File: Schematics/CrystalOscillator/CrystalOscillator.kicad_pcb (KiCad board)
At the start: 2 copper layers, 8 parts, among them J1 Conn_01x24_Female, U1 74HC14, Y1 4MHz Crystal

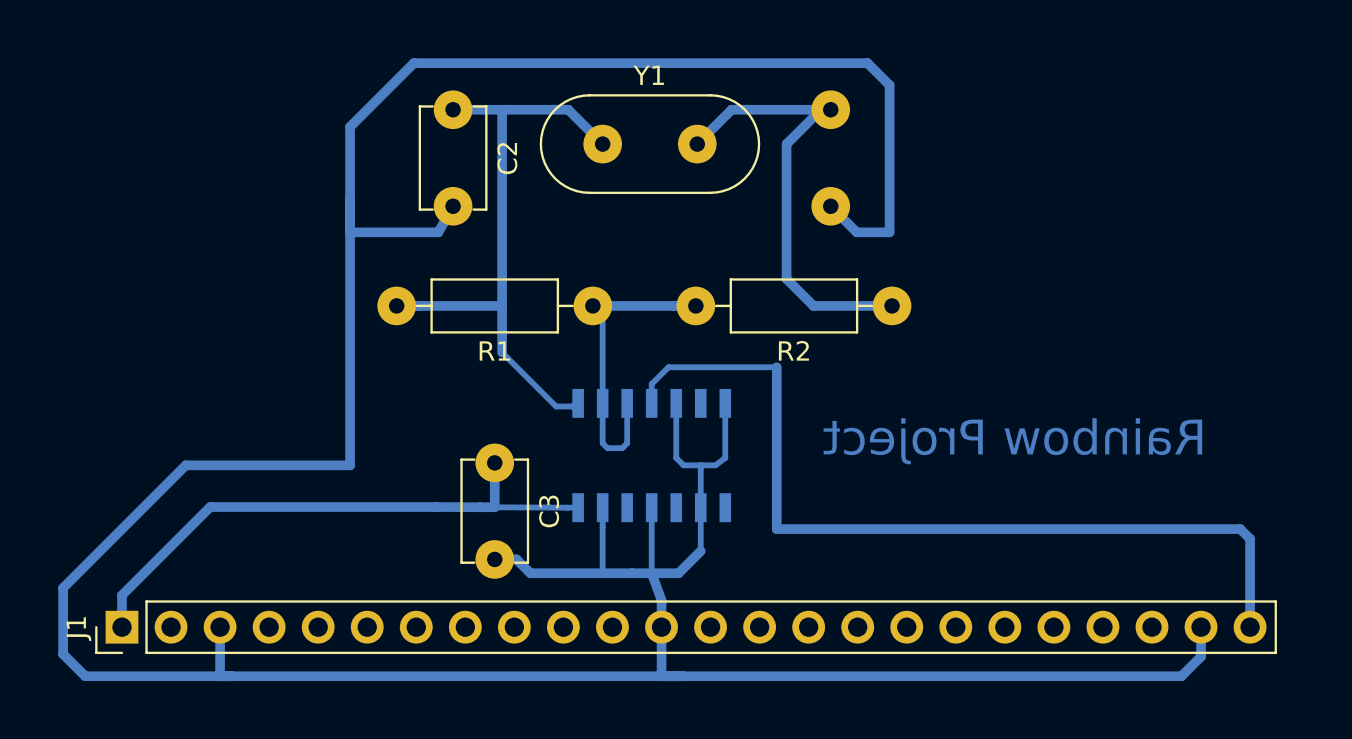
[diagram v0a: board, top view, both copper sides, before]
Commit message: Final version of 4 MHz clock PCB
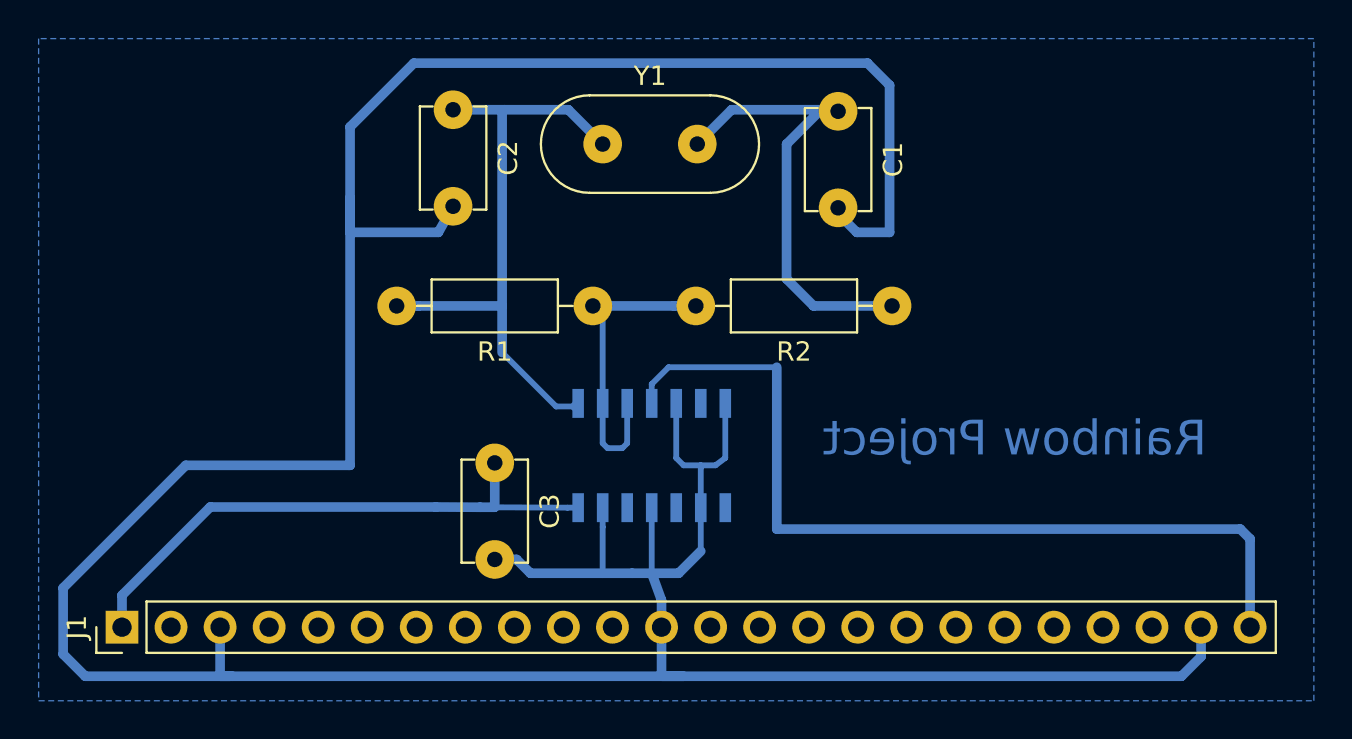
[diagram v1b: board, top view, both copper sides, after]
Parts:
- C1: moved to F.Cu
- moved C1 0.39 mm to (163.3, 104.1)
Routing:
- added copper zone on B.Cu, net GND
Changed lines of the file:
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@@
     (visible_elements 7FFFFFFF)
     (pcbplotparams
-      (layerselection 0x010fc_ffffffff)
+      (layerselection 0x00000_fffffffe)
       (usegerberextensions false)
       (usegerberattributes false)
@@
       (psa4output false)
       (plotreference true)
-      (plotvalue true)
-      (plotinvisibletext false)
+      (plotvalue false)
+      (plotinvisibletext true)
       (padsonsilk false)
       (subtractmaskfromsilk false)
-      (outputformat 1)
+      (outputformat 4)
       (mirror false)
       (drillshape 1)
       (scaleselection 1)
-      (outputdirectory ""))
+      (outputdirectory "D:/Data/Desktop/"))
   )
   (net 0 "")
@@
     )
   )
-  (module Capacitor_THT:C_Disc_D5.1mm_W3.2mm_P5.00mm (layer B.Cu)
-    (at 162.941 104.013 270)
+  (module Capacitor_THT:C_Disc_D5.1mm_W3.2mm_P5.00mm (layer F.Cu)
+    (at 163.322 104.093 270)
     (descr "C, Disc series, Radial, pin pitch=5.00mm, , diameter*width=5.1*3.2mm^2, Capacitor, http://www.vishay.com/docs/45233/krseries.pdf")
     (tags "C Disc series Radial pin pitch 5.00mm  diameter 5.1mm width 3.2mm Capacitor")
-    (fp_text reference C1 (at 2.5 2.85 270) (layer B.SilkS)
-      (effects (font (size 1 1) (thickness 0.15)) (justify mirror))
-    )
-    (fp_text value 3.3p (at 2.5 -2.85 270) (layer B.Fab)
-      (effects (font (size 1 1) (thickness 0.15)) (justify mirror))
-    )
-    (fp_line (start -0.05 1.6) (end -0.05 -1.6) (layer B.Fab) (width 0.1))
-    (fp_line (start -0.05 -1.6) (end 5.05 -1.6) (layer B.Fab) (width 0.1))
-    (fp_line (start 5.05 -1.6) (end 5.05 1.6) (layer B.Fab) (width 0.1))
-    (fp_line (start 5.05 1.6) (end -0.05 1.6) (layer B.Fab) (width 0.1))
-    (fp_line (start -0.17 1.721) (end 5.17 1.721) (layer B.SilkS) (width 0.12))
-    (fp_line (start -0.17 -1.721) (end 5.17 -1.721) (layer B.SilkS) (width 0.12))
-    (fp_line (start -0.17 1.721) (end -0.17 1.055) (layer B.SilkS) (width 0.12))
-    (fp_line (start -0.17 -1.055) (end -0.17 -1.721) (layer B.SilkS) (width 0.12))
-    (fp_line (start 5.17 1.721) (end 5.17 1.055) (layer B.SilkS) (width 0.12))
-    (fp_line (start 5.17 -1.055) (end 5.17 -1.721) (layer B.SilkS) (width 0.12))
-    (fp_line (start -1.05 1.85) (end -1.05 -1.85) (layer B.CrtYd) (width 0.05))
-    (fp_line (start -1.05 -1.85) (end 6.05 -1.85) (layer B.CrtYd) (width 0.05))
-    (fp_line (start 6.05 -1.85) (end 6.05 1.85) (layer B.CrtYd) (width 0.05))
-    (fp_line (start 6.05 1.85) (end -1.05 1.85) (layer B.CrtYd) (width 0.05))
-    (fp_text user %R (at 2.54 -0.381 270) (layer B.Fab)
-      (effects (font (size 1 1) (thickness 0.15)) (justify mirror))
+    (fp_text reference C1 (at 2.5 -2.85 270) (layer F.SilkS)
+      (effects (font (size 1 1) (thickness 0.15)))
+    )
+    (fp_text value 3.3p (at 2.5 2.85 270) (layer F.Fab)
+      (effects (font (size 1 1) (thickness 0.15)))
+    )
+    (fp_line (start -0.05 -1.6) (end -0.05 1.6) (layer F.Fab) (width 0.1))
+    (fp_line (start -0.05 1.6) (end 5.05 1.6) (layer F.Fab) (width 0.1))
+    (fp_line (start 5.05 1.6) (end 5.05 -1.6) (layer F.Fab) (width 0.1))
+    (fp_line (start 5.05 -1.6) (end -0.05 -1.6) (layer F.Fab) (width 0.1))
+    (fp_line (start -0.17 -1.721) (end 5.17 -1.721) (layer F.SilkS) (width 0.12))
+    (fp_line (start -0.17 1.721) (end 5.17 1.721) (layer F.SilkS) (width 0.12))
+    (fp_line (start -0.17 -1.721) (end -0.17 -1.055) (layer F.SilkS) (width 0.12))
+    (fp_line (start -0.17 1.055) (end -0.17 1.721) (layer F.SilkS) (width 0.12))
+    (fp_line (start 5.17 -1.721) (end 5.17 -1.055) (layer F.SilkS) (width 0.12))
+    (fp_line (start 5.17 1.055) (end 5.17 1.721) (layer F.SilkS) (width 0.12))
+    (fp_line (start -1.05 -1.85) (end -1.05 1.85) (layer F.CrtYd) (width 0.05))
+    (fp_line (start -1.05 1.85) (end 6.05 1.85) (layer F.CrtYd) (width 0.05))
+    (fp_line (start 6.05 1.85) (end 6.05 -1.85) (layer F.CrtYd) (width 0.05))
+    (fp_line (start 6.05 -1.85) (end -1.05 -1.85) (layer F.CrtYd) (width 0.05))
+    (fp_text user %R (at 2.54 0.381 270) (layer F.Fab)
+      (effects (font (size 1 1) (thickness 0.15)))
     )
     (pad 1 thru_hole circle (at 0 0 270) (size 2 2) (drill 0.8) (layers *.Cu *.Mask)
@@
   (segment (start 156.21 124.62) (end 156.21 126.873) (width 0.3) (layer B.Cu) (net 5))
   (segment (start 153.67 124.62) (end 153.67 128.016) (width 0.3) (layer B.Cu) (net 5))
-  (segment (start 156.21 122.555) (end 156.21 124.62) (width 0.3) (layer B.Cu) (net 5))
   (segment (start 154.178 129.413) (end 154.178 130.81) (width 0.5) (layer B.Cu) (net 5))
   (segment (start 153.67 128.016) (end 154.178 129.413) (width 0.5) (layer B.Cu) (net 5))
   (segment (start 145.542 127.301) (end 145.622 127.381) (width 0.5) (layer B.Cu) (net 5))
-  (segment (start 156.21 122.428) (end 156.21 122.555) (width 0.3) (layer B.Cu) (net 5))
   (segment (start 155.321 122.428) (end 156.21 122.428) (width 0.3) (layer B.Cu) (net 5))
-  (segment (start 154.94 119.22) (end 154.94 122.047) (width 0.3) (layer B.Cu) (net 5))
   (segment (start 154.94 122.047) (end 155.321 122.428) (width 0.3) (layer B.Cu) (net 5))
   (segment (start 156.972 122.428) (end 156.21 122.428) (width 0.3) (layer B.Cu) (net 5))
-  (segment (start 157.48 119.22) (end 157.48 122.047) (width 0.3) (layer B.Cu) (net 5))
   (segment (start 157.48 122.047) (end 156.972 122.428) (width 0.3) (layer B.Cu) (net 5))
   (segment (start 152.654 128.016) (end 153.67 128.016) (width 0.5) (layer B.Cu) (net 5))
@@
   (segment (start 131.826 133.35) (end 124.333 133.35) (width 0.5) (layer B.Cu) (net 5))
   (segment (start 124.333 133.35) (end 123.19 132.207) (width 0.5) (layer B.Cu) (net 5))
+  (segment (start 156.21 122.555) (end 156.21 124.62) (width 0.3) (layer B.Cu) (net 5))
+  (segment (start 156.21 122.428) (end 156.21 122.555) (width 0.3) (layer B.Cu) (net 5))
+  (segment (start 157.48 119.22) (end 157.48 122.047) (width 0.3) (layer B.Cu) (net 5))
+  (segment (start 154.94 119.22) (end 154.94 122.047) (width 0.3) (layer B.Cu) (net 5))
   (segment (start 149.86 124.62) (end 149.31 124.62) (width 0.3) (layer B.Cu) (net 10))
   (segment (start 149.31 124.62) (end 144.78 124.598067) (width 0.3) (layer B.Cu) (net 10))
@@
   (segment (start 144.78 124.598067) (end 142.494 124.587) (width 0.5) (layer B.Cu) (net 10))
   (segment (start 142.494 124.587) (end 130.81 124.587) (width 0.5) (layer B.Cu) (net 10))
+  (zone (net 5) (net_name GND) (layer B.Cu) (hatch edge 0.508)
+    (connect_pads (clearance 1.5))
+    (min_thickness 0.254)
+    (fill yes (arc_segments 32) (thermal_gap 1.5) (thermal_bridge_width 0.508) (smoothing fillet))
+    (polygon
+      (pts
+        (xy 121.92 100.33) (xy 121.92 134.62) (xy 187.96 134.62) (xy 187.96 100.33)
+      )
+    )
+  )
 )
